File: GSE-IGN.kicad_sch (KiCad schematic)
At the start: 34 parts, among them J1 Conn_01x02, J2 LD1117S50, J3 debug-sw1, J4 RJ45, J5 Igniter-1, J6 debug-sw1, J7 Igniter-2, J8 RJ45, J9 Conn_01x04_Socket, Q1 BSS138, U1 ATMEGA328P-PU, U3 TLP3543A

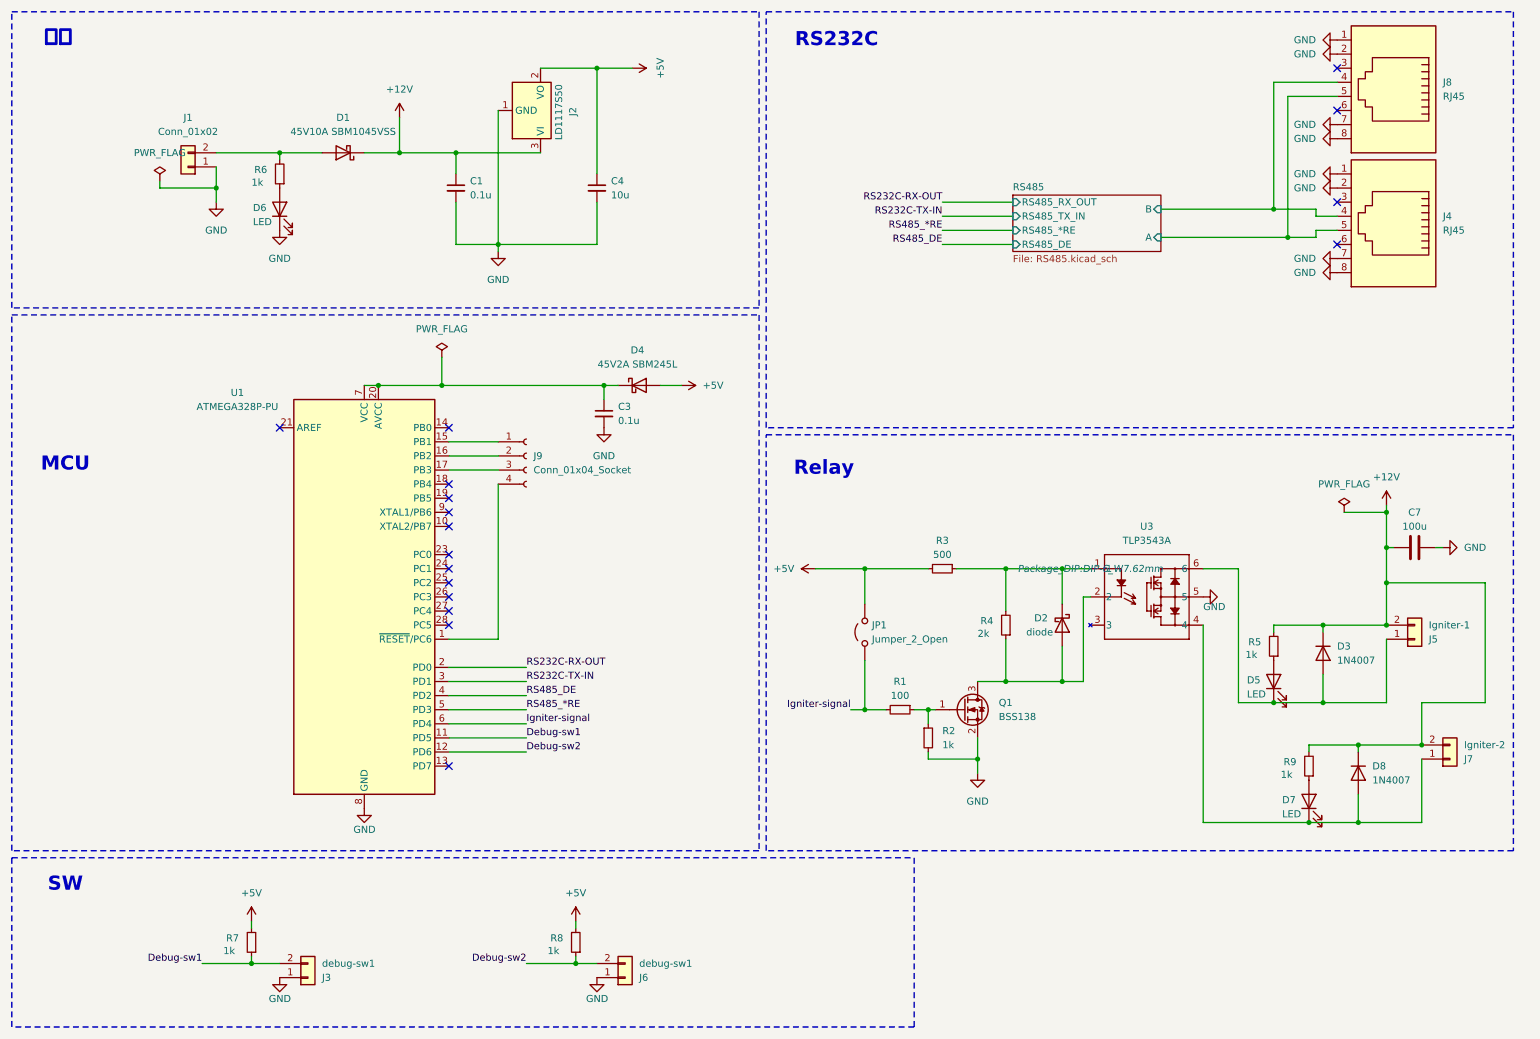
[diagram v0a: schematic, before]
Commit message: アートワーク終わり
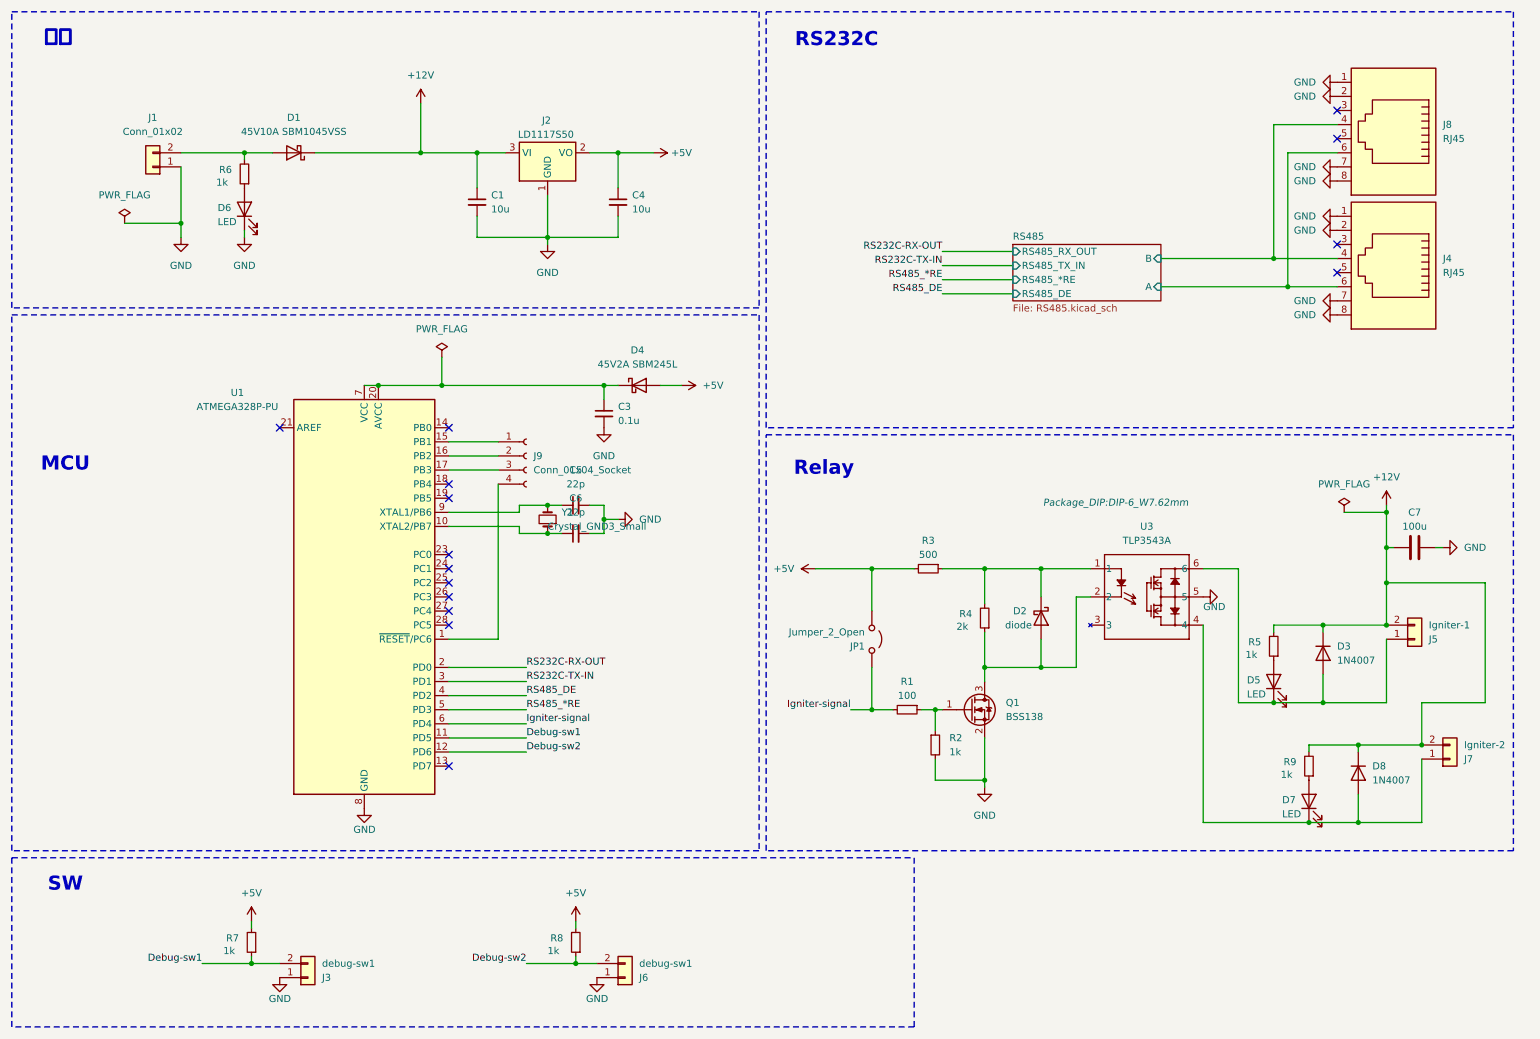
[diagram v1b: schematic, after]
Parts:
- added C5, C6: 22p, Capacitor_SMD:C_0603_1608Metric, symbol Device:C_Small
- added Y1: Crystal_GND3_Small, Crystal:Crystal_HC49-4H_Vertical, symbol Device:Crystal_Small
- C1: value 0.1u -> 10u; footprint Diode_SMD:D_0402_1005Metric -> Capacitor_THT:CP_Radial_D4.0mm_P1.50mm
- J4, J8: footprint Connector_RJ:RJ45_Wuerth_7499010211A_Horizontal -> 0000_my_footprint:78108P8C
- J9: footprint Connector_PinSocket_1.00mm:PinSocket_1x04_P1.00mm_Vertical -> Connector_PinSocket_2.54mm:PinSocket_1x04_P2.54mm_Vertical
- JP1: footprint Connector_PinSocket_2.54mm:PinSocket_1x02_P2.54mm_Vertical -> Connector_JST:JST_XH_B2B-XH-A_1x02_P2.50mm_Vertical
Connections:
- net +5V: now also JP1.1 (A); no longer JP1.2 (B)
- net GND: now also C5.2, C6.2
- net Igniter-signal: now also JP1.2 (B); no longer JP1.1 (A)
- net RS485/A: now also J4.6, J8.6; no longer J4.5, J8.5
- net at U1.10 (XTAL2/PB7): now also C6.1, Y1.1
- net at U1.9 (XTAL1/PB6): now also C5.1, Y1.2
- no-connect marks 17 -> 15
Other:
- moved on the sheet: C1, C4, D1, D2, D6, J1, J2, J4, J8, JP1, Q1, R1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
